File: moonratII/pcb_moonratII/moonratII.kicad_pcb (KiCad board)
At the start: 2 copper layers, 108 x 65 mm, 34 parts, among them J1 Barrel_Jack_Switch_SMT, J10 Conn_02x05_Odd_Even, J11 Screw_Terminal_01x02, J2 HS96L03W2C03_0.96_Oled, J5 Conn_02x05_Odd_Even, J6 Screw_Terminal_01x06, J9 Screw_Terminal_01x06, Q1 IRF520N, Q2 BSS138, SW1 6mm 2 Pin Tact NO Breadboard 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, SW2 6mm 2 Pin Tact NO Breadboard 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, SW3 6mm 2 Pin Tact NO Breadboard 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, U1 TMP36GRTZ-REEL7

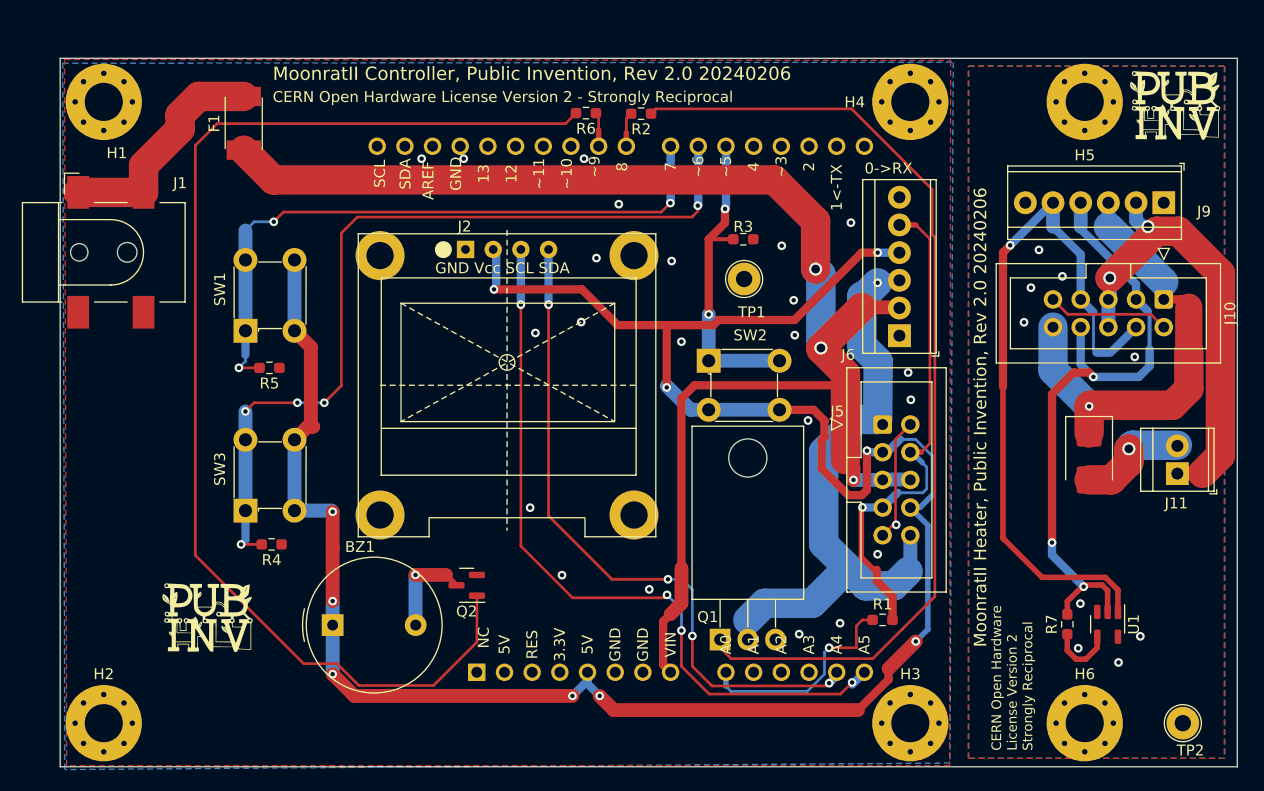
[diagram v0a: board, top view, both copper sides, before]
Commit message: Clean up some via spacing and ground pours.
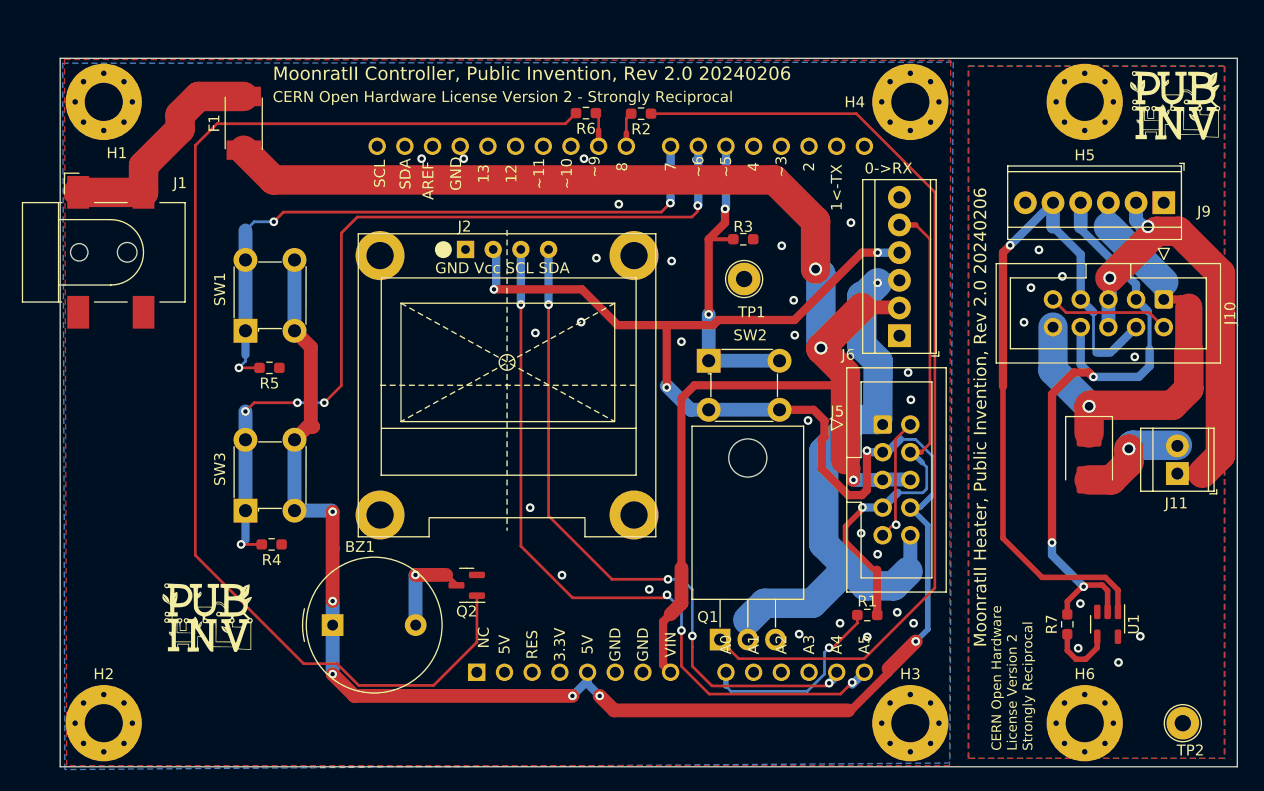
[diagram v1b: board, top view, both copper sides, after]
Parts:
- moved R1 1.47 mm to (124.0, 136.1)
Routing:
- net TEMP_IN: track 20.0 -> 18.0 mm
- net HEATER_ON: track 89.7 -> 88.5 mm
- net GND: vias 23 -> 27
